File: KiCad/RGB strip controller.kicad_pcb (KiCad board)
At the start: 2 copper layers, 17.1 x 48.9 mm, 16 parts, among them J1 USB_C_Receptacle_USB2.0, J2 Conn_01x03, SW1 SW_SPST, U1 ESP-01, U2 LM317_TO-220

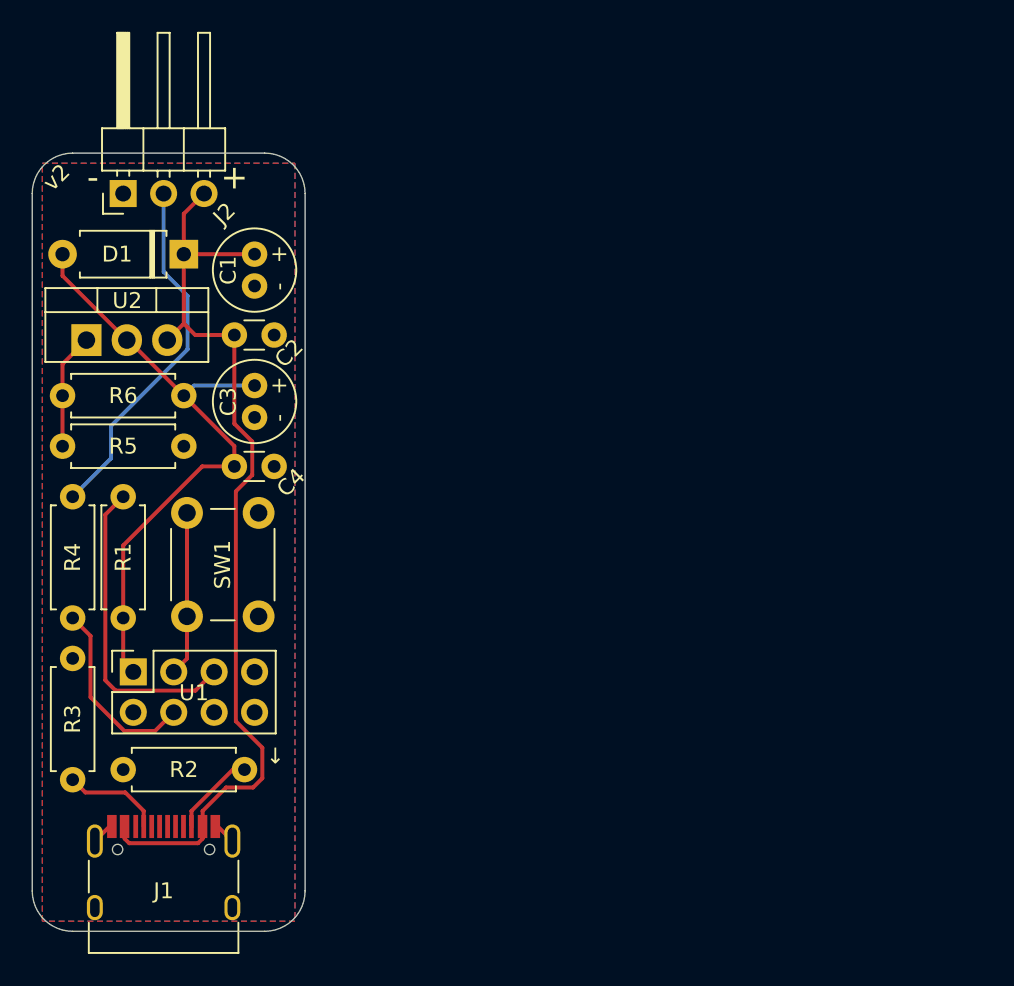
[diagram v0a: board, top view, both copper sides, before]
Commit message: PCB v3
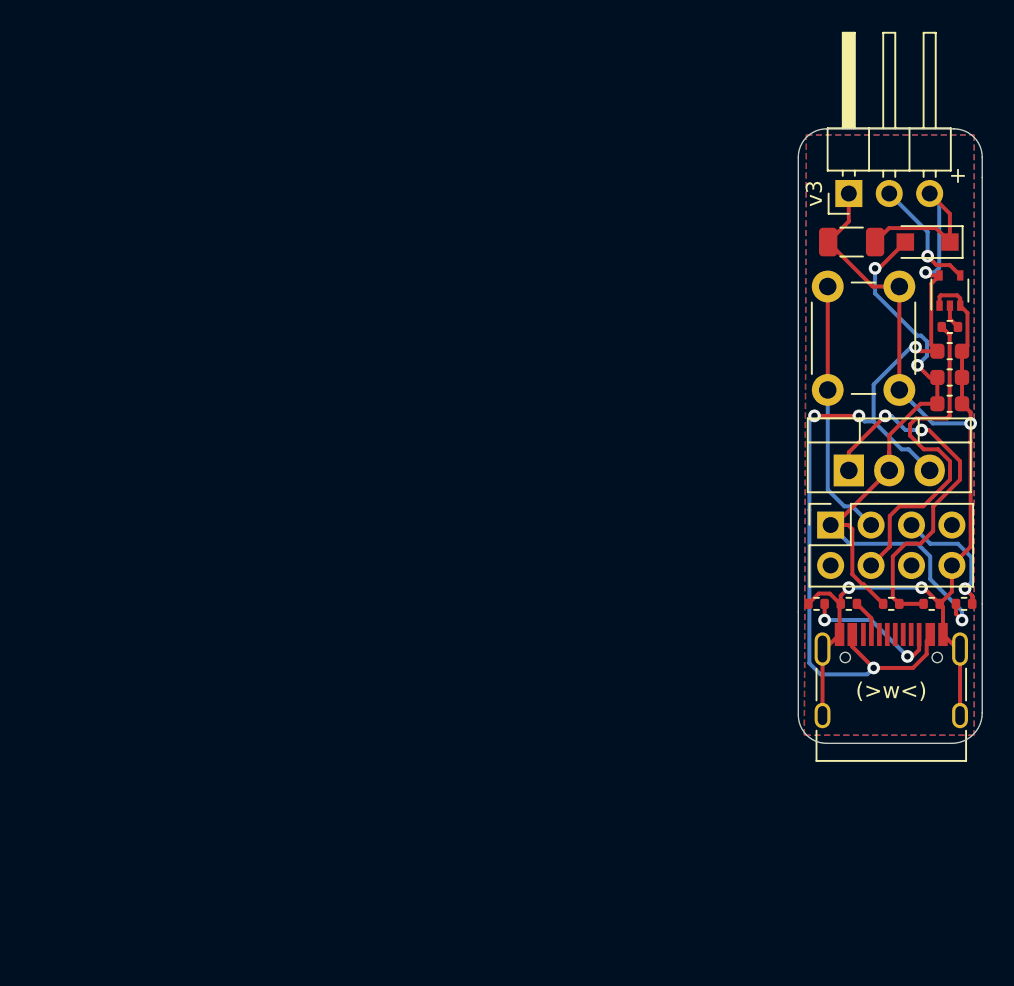
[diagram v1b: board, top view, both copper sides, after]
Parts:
- added U3: TC7SZ125FU, Package_TO_SOT_SMD:SOT-353_SC-70-5, F.Cu at (182.8, 68.3)
- C1: footprint Capacitor_THT:C_Radial_D5.0mm_H11.0mm_P2.00mm -> Capacitor_SMD:C_1206_3216Metric
- C2, C4: footprint Capacitor_THT:C_Disc_D3.0mm_W1.6mm_P2.50mm -> Capacitor_SMD:C_0603_1608Metric
- C3: footprint Capacitor_THT:C_Radial_D5.0mm_H11.0mm_P2.00mm -> Capacitor_SMD:C_0603_1608Metric
- D1: footprint Diode_THT:D_A-405_P7.62mm_Horizontal -> Diode_SMD:D_SOD-123F
- R1, R2, R3, R4, R5, R6: footprint Resistor_THT:R_Axial_DIN0207_L6.3mm_D2.5mm_P7.62mm_Horizontal -> Resistor_SMD:R_0402_1005Metric
- moved R4 56.1 mm to (182.8, 70.6), turned to 180 degrees
- moved R5 55.5 mm to (181.6, 88.0)
- moved R1 53.3 mm to (183.6, 88.0), turned to 180 degrees
- moved R3 50.0 mm to (176.4, 88.0), turned to 180 degrees
- moved U2 48.6 mm to (176.4, 79.6)
- moved J1 47.3 mm to (179.1, 94.0)
- moved D1 46.7 mm to (181.4, 65.3)
- moved R6 46.3 mm to (179.1, 88.0), turned to 0 degrees
- moved J2 45.6 mm to (176.4, 62.2)
- moved C4 45.1 mm to (182.7, 75.4)
- moved C2 45.0 mm to (182.7, 72.1)
- moved U1 44.8 mm to (175.3, 83.1)
- moved C3 43.7 mm to (182.7, 73.8), turned to 0 degrees
- moved SW1 42.7 mm to (179.6, 68.1)
- moved C1 37.5 mm to (176.6, 65.3), turned to 180 degrees
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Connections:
- J2 pad 2: LED_Data -> Net-(J2-Pad2)
- R4 pad 1: LED_Data -> Net-(R4-Pad1)
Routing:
- net GND: track 2.90 -> 69.4 mm, vias 0 -> 3
- net LED_Data: track 22.7 -> 0.00 mm
- net Net-(R5-Pad1): track 7.29 -> 23.3 mm, vias 0 -> 2
- net Net-(R1-Pad1): track 19.6 -> 7.97 mm, vias 0 -> 1
- net Net-(R4-Pad2): track 12.0 -> 21.9 mm
- net Net-(J2-Pad2): track 0.00 -> 7.48 mm, vias 0 -> 1
- net +3V3: track 39.8 -> 46.8 mm, vias 0 -> 3
- net Net-(SW1-Pad2): track 10.3 -> 16.4 mm
- net +5V: track 59.8 -> 64.8 mm, vias 0 -> 5
- net Net-(J1-PadA5): track 6.25 -> 2.30 mm
- net Net-(J1-PadB5): track 5.38 -> 9.09 mm, vias 0 -> 2
- net Net-(R4-Pad1): track 0.00 -> 1.55 mm
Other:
- board size 17.1 x 48.9 mm -> 11.6 x 38.6 mm
- board text added: "(>w<)"
- board text added: "actually 300 and 470"
- board text added: "v3"
- board text removed: "-"
- board text removed: "v2"
- board text removed: "←"
